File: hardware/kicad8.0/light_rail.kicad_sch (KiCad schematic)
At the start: 209 parts, among them J1 USB_C_Receptacle_USB2.0_16P, J2 Conn_01x04_Pin, J3 AVR-ISP-6, SW1 SW_Push, SW10 SW_Push, SW11 SW_Push, SW12 SW_Push, SW13 SW_Push, SW14 SW_SPST, SW2 SW_Push, SW3 SW_Push, SW4 SW_Push, SW5 SW_Push, SW6 SW_Push, SW7 SW_Push, SW8 SW_Push, SW9 SW_Push, U1 ATmega32U4-A, U2 IS31FL3731-SA, U3 AS1115-BSST, U4 MIC5219-3.3YM5, U5 KCSC02-105, U6 KCSC02-105, U7 KCSC02-105, X1 ECS-2520MV-xxx-xx

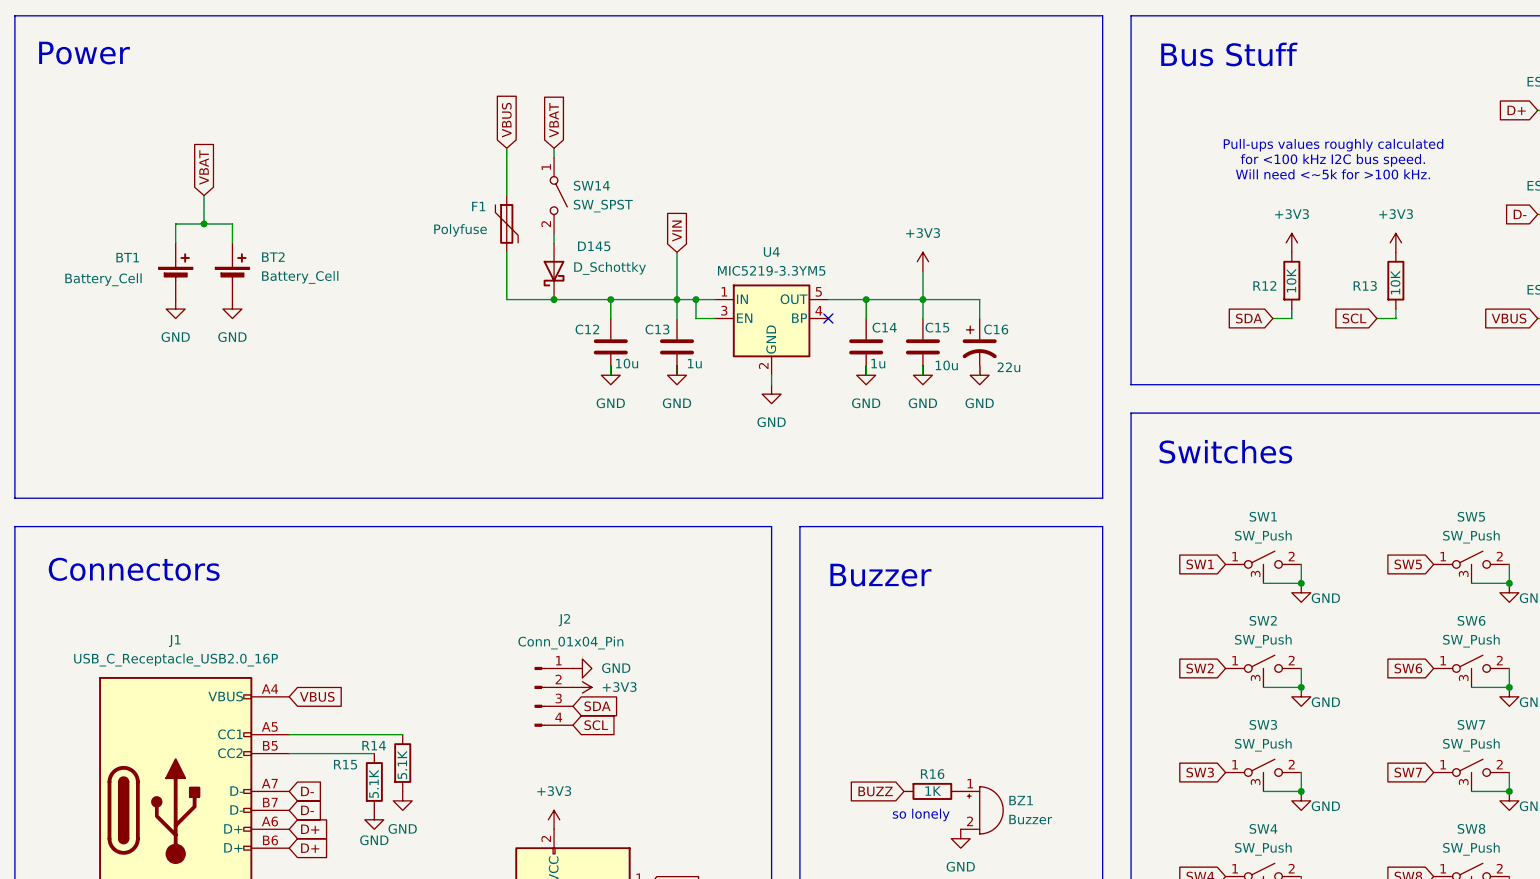
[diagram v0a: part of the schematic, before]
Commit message: fab updates 2
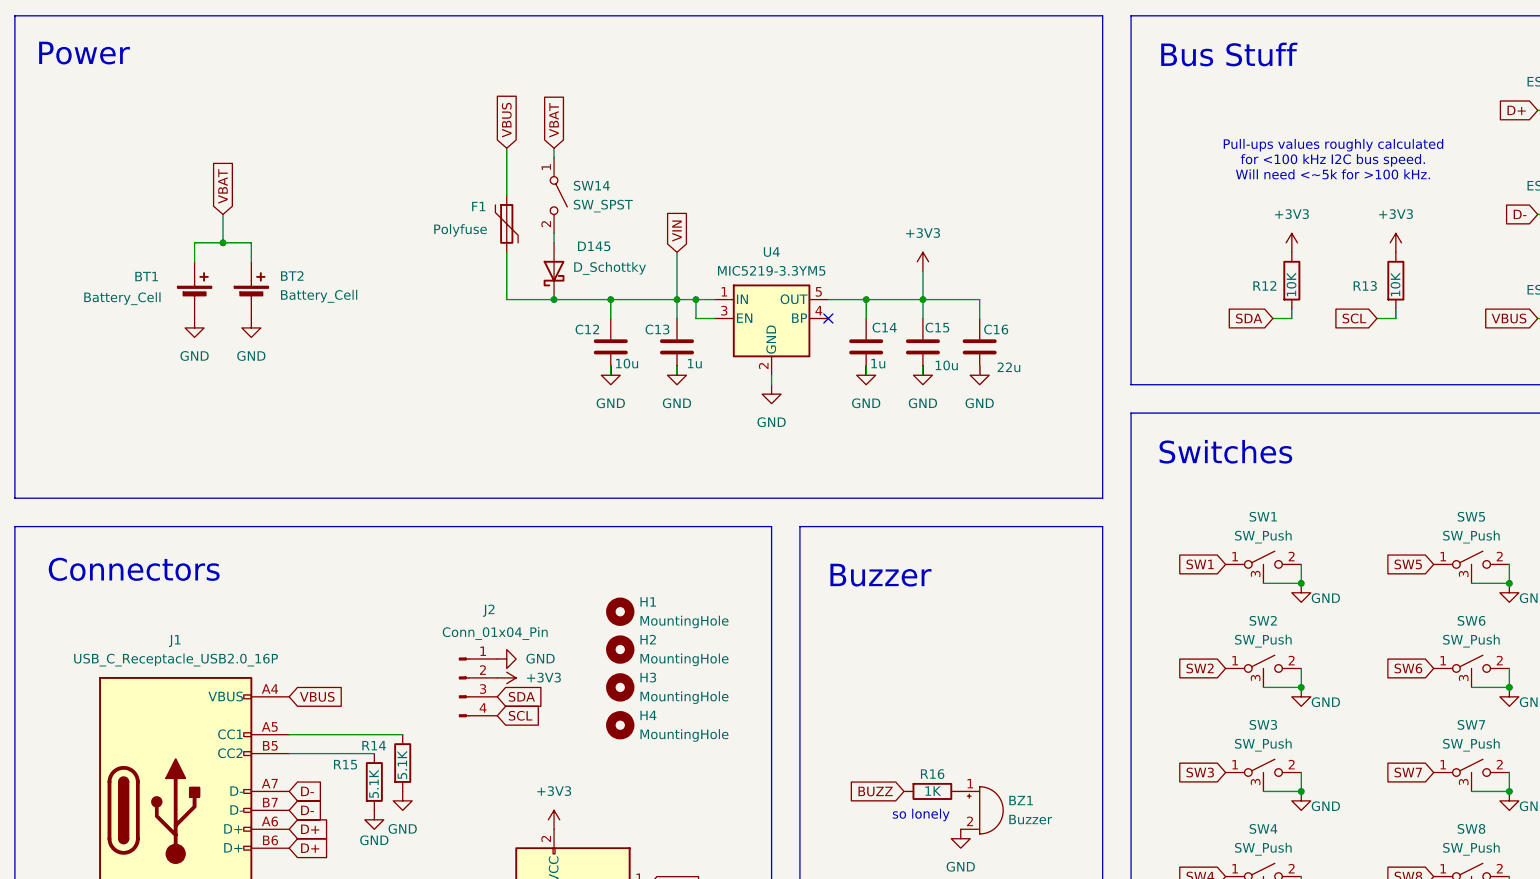
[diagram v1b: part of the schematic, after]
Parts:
- added H1, H2, H3, H4: MountingHole, Light_Rail:MountingHole_Custom, symbol Mechanical:MountingHole
- C16: symbol Device:C_Polarized_US -> Device:C
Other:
- moved on the sheet: BT1, BT2, J2
